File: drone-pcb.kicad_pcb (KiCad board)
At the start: 2 copper layers, 65 x 48.5 mm, 47 parts, among them J1 Conn_01x02_Pin, J10 Conn_01x03_Pin, J11 Conn_01x03_Pin, J12 Conn_01x03_Pin, J2 Conn_01x02_Pin, J3 Conn_01x02_Pin, J4 Conn_01x02_Pin, J5 Conn_01x02_Pin, J6 Conn_01x02_Pin, J7 USB_C_Receptacle_USB2.0_16P, J8 Conn_01x02_Pin, J9 Conn_01x03_Pin, Q1 AO3400A, Q2 AO3400A, Q3 AO3400A, Q4 AO3400A, Q5 AO3400A, Q6 AO3400A, SW1 CK_KMS2xxGP, U1 STM32F030C8Tx, U2 nRF24L01P, U3 MCP73831-2-OT, U4 TLV75533PDBV, U5 MPU-6050

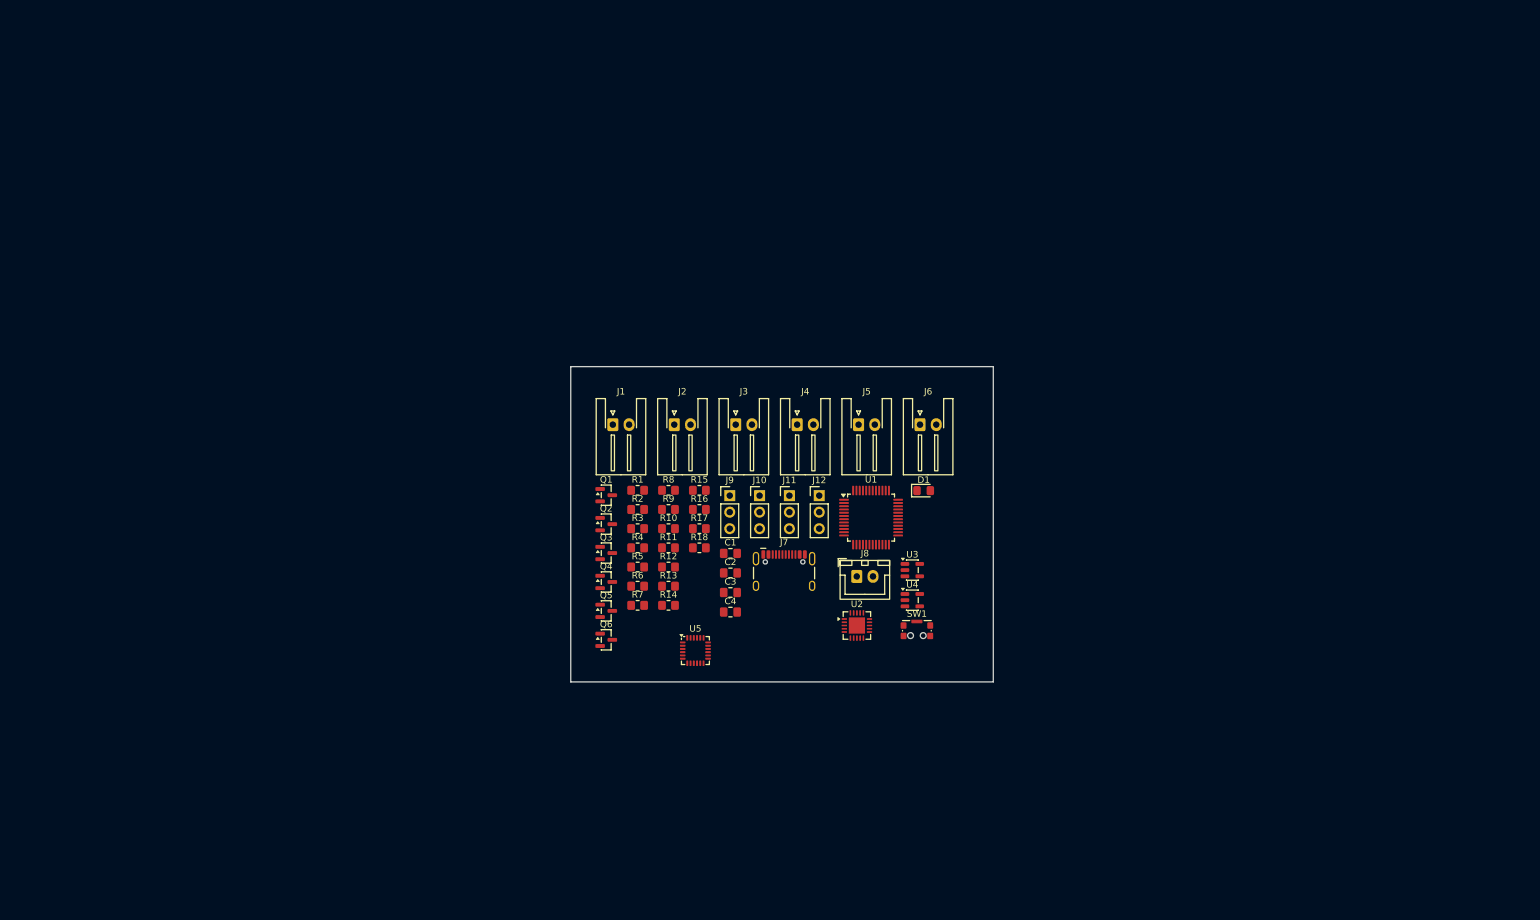
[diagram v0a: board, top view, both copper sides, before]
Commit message: start placing footprints
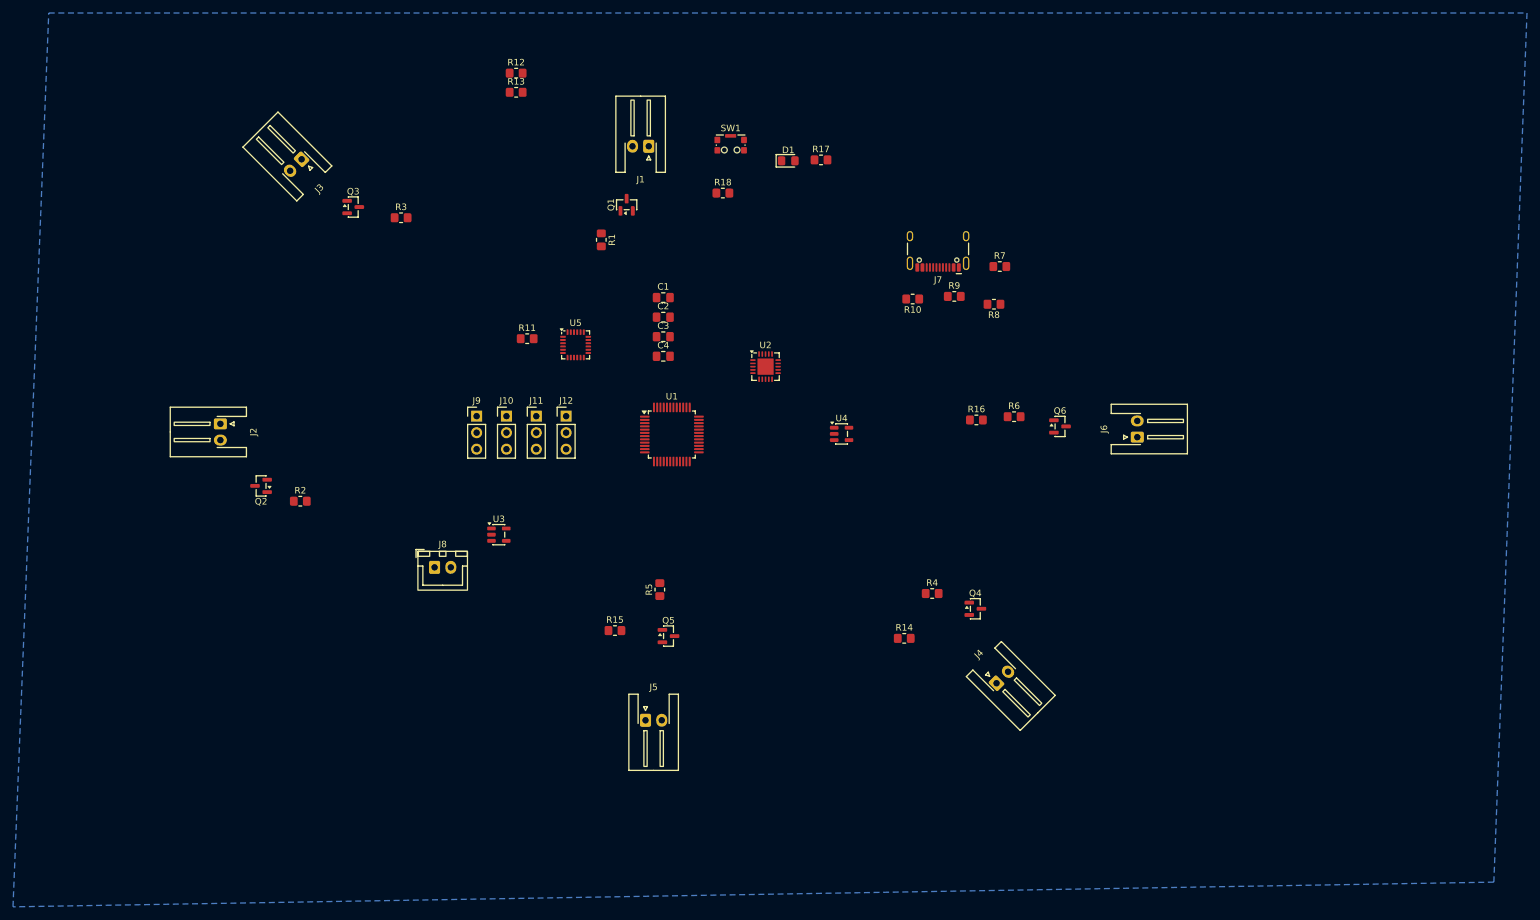
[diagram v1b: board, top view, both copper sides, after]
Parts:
- moved SW1 80.0 mm to (147.6, 42.9)
- moved R13 79.5 mm to (114.6, 34.8)
- moved R12 79.5 mm to (114.6, 31.9)
- moved J3 78.3 mm to (81.6, 45.1), turned to -135 degrees
- moved Q6 77.1 mm to (198.3, 86.2)
- moved R7 76.3 mm to (189.0, 61.6)
- moved J2 69.8 mm to (69.1, 85.8), turned to -90 degrees
- moved Q3 65.9 mm to (89.5, 52.5)
- moved J8 65.0 mm to (102.0, 107.9)
- moved U3 63.8 mm to (111.9, 102.8)
- moved R6 63.5 mm to (191.2, 84.7)
- moved R3 60.1 mm to (96.9, 54.1)
- moved R17 59.7 mm to (161.5, 45.2)
- moved R8 57.7 mm to (188.1, 67.4), turned to 180 degrees
- moved Q4 56.9 mm to (185.2, 114.2)
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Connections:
- U5 pad 1: unconnected-(U5-CLKIN-Pad1) -> GND
- U5 pad 12: unconnected-(U5-INT-Pad12) -> /imu_INT
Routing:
- added copper zone on B.Cu, net GND
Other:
- board outline removed
